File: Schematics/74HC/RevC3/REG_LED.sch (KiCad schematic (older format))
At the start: 224 parts

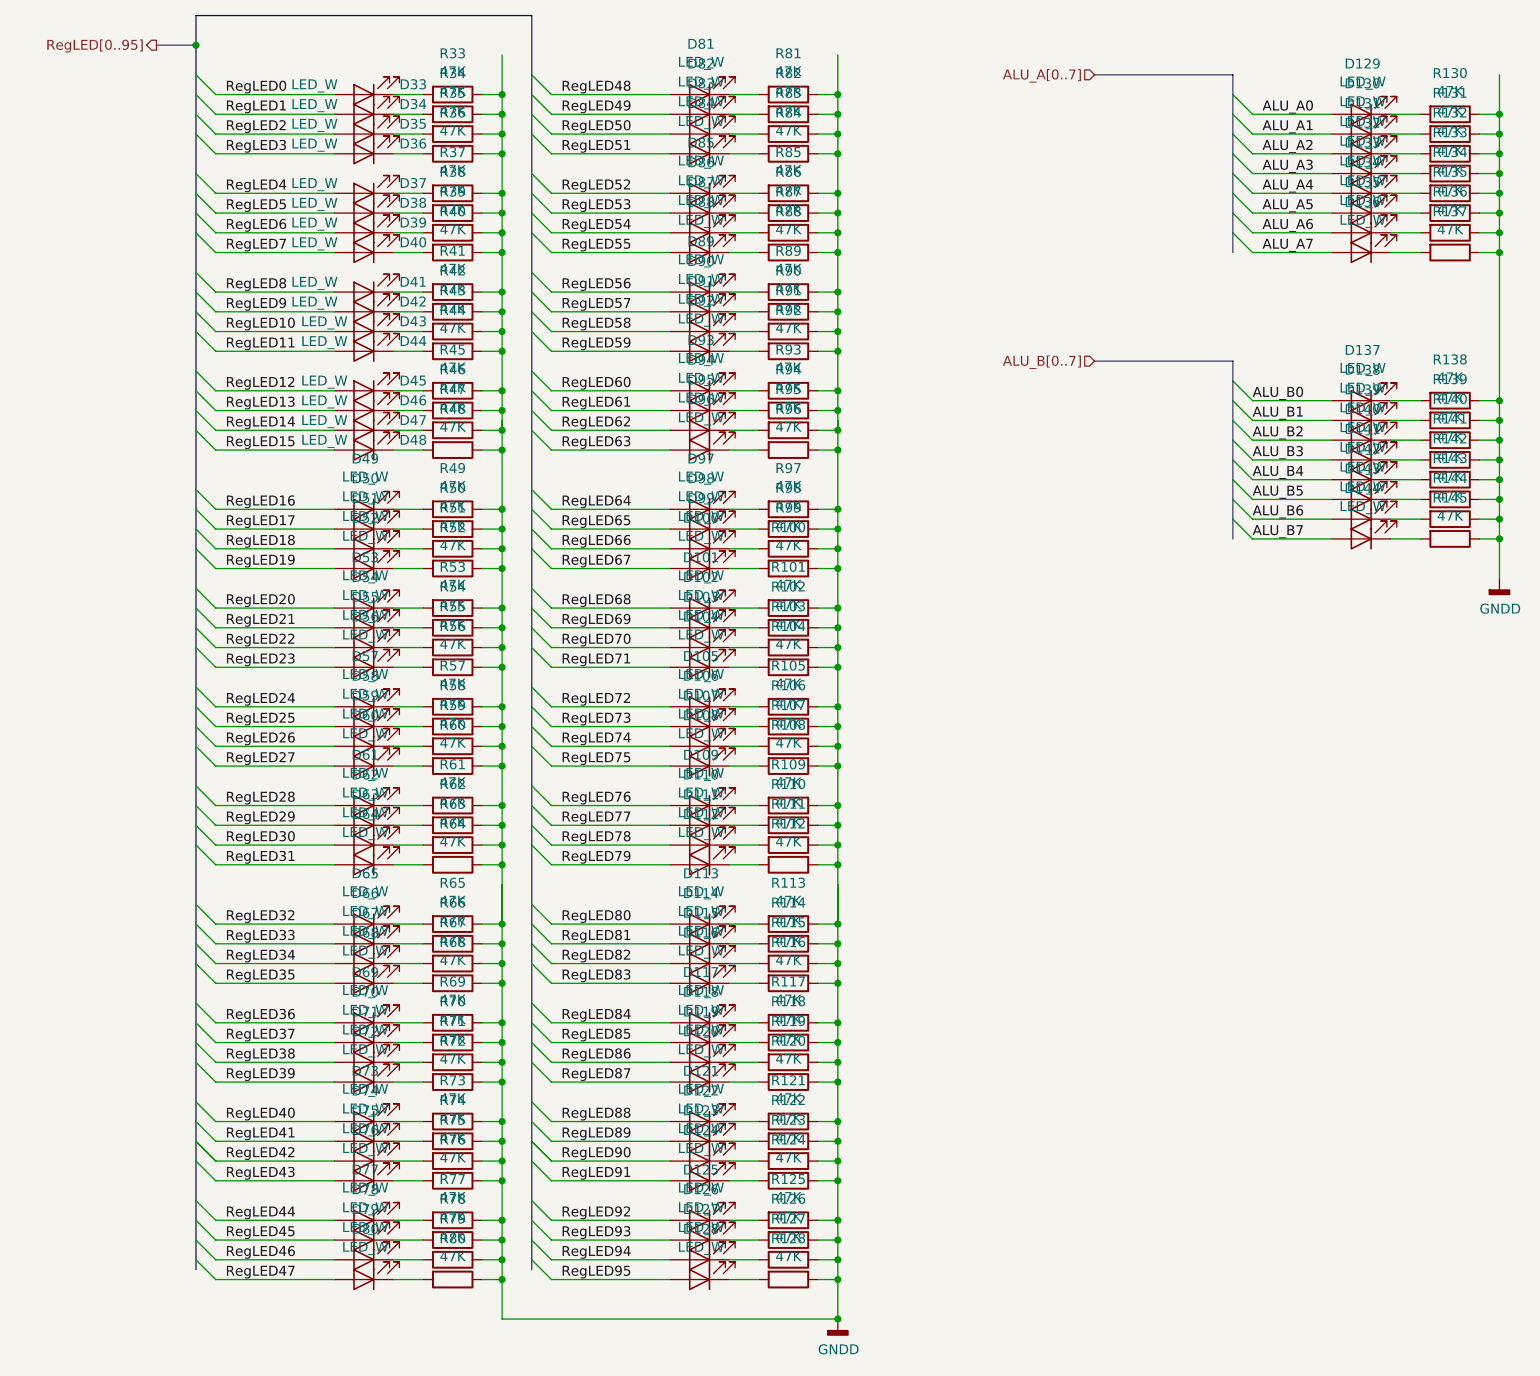
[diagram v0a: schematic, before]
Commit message: revA3
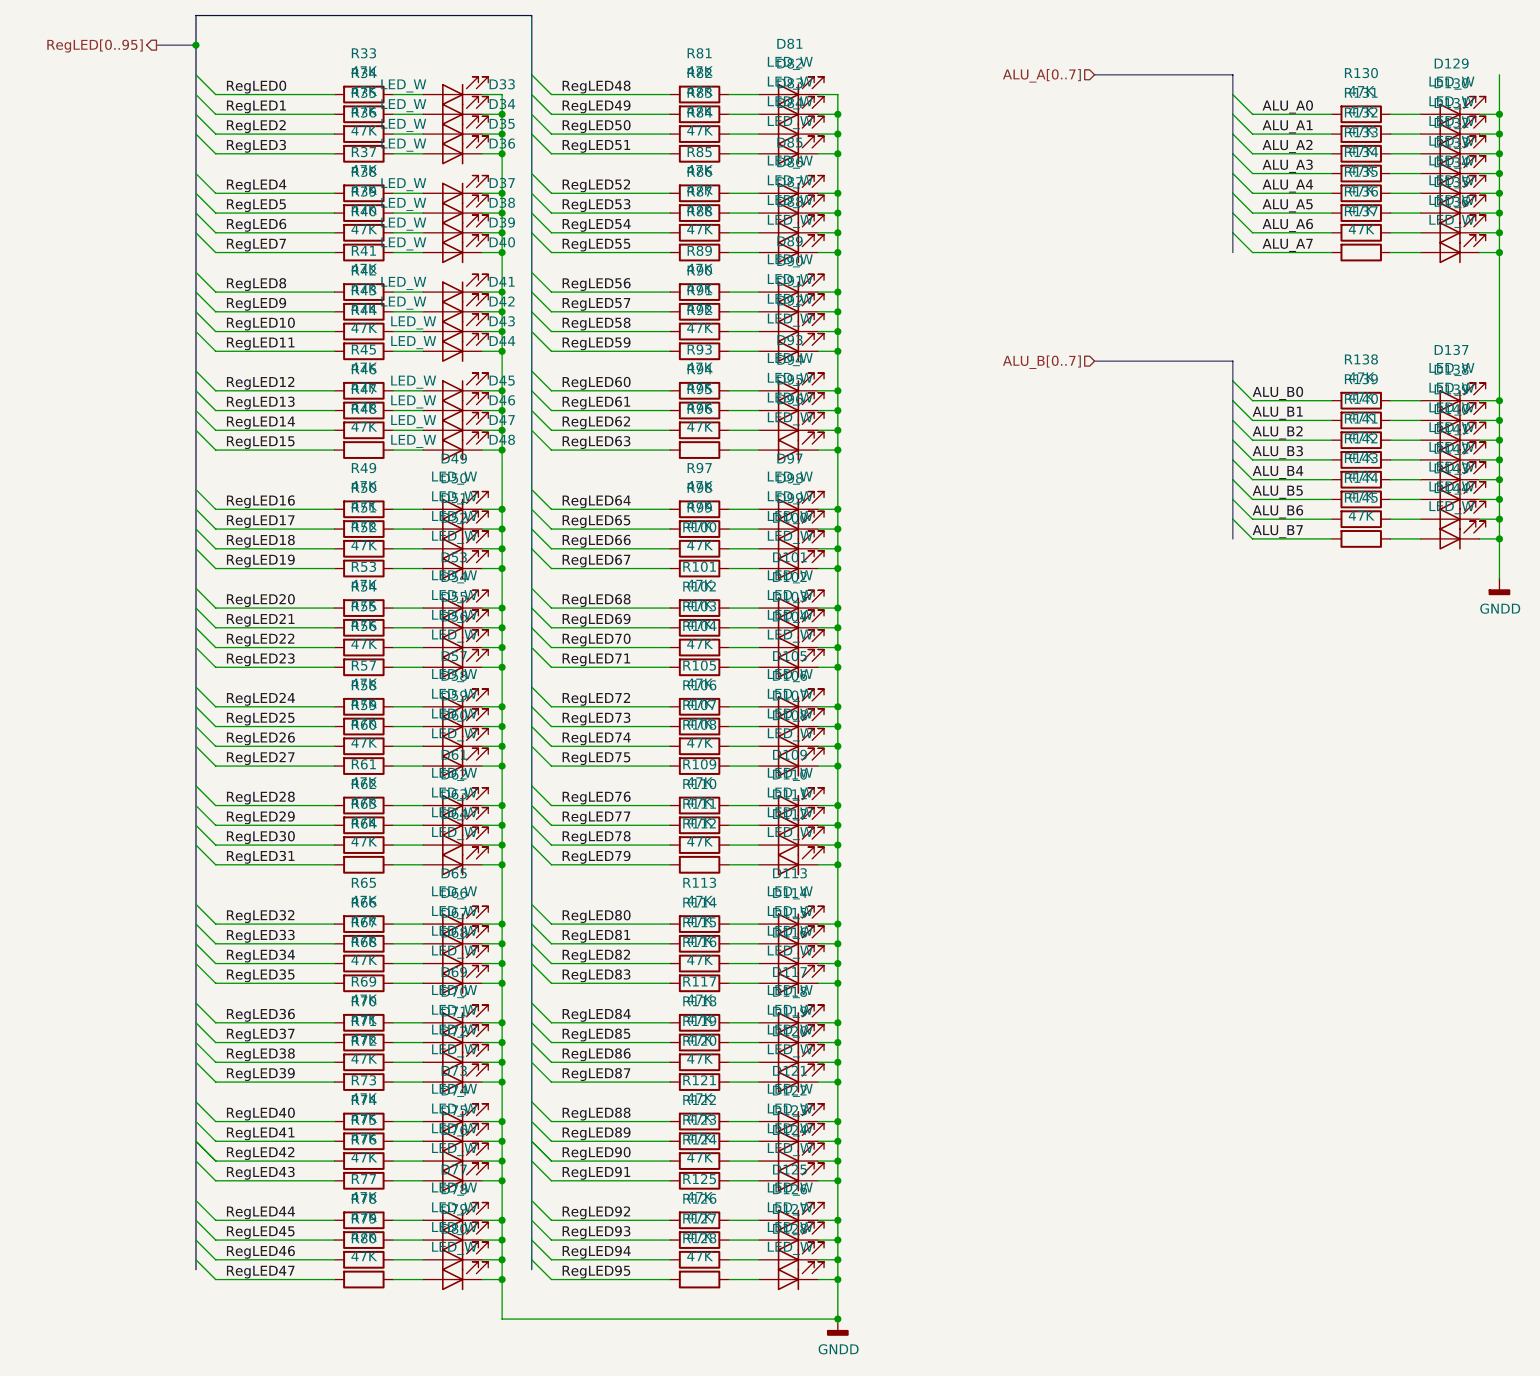
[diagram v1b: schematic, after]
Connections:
- net ALU_A0: now also R130.2; no longer D129.2 (A)
- net ALU_A1: now also R131.2; no longer D130.2 (A)
- net ALU_A2: now also R132.2; no longer D131.2 (A)
- net ALU_A3: now also R133.2; no longer D132.2 (A)
- net ALU_A4: now also R134.2; no longer D133.2 (A)
- net ALU_A5: now also R135.2; no longer D134.2 (A)
- net ALU_A6: now also R136.2; no longer D135.2 (A)
- net ALU_A7: now also R137.2; no longer D136.2 (A)
- net ALU_B0: now also R138.2; no longer D137.2 (A)
- net ALU_B1: now also R139.2; no longer D138.2 (A)
- net ALU_B2: now also R140.2; no longer D139.2 (A)
- net ALU_B3: now also R141.2; no longer D140.2 (A)
- net ALU_B4: now also R142.2; no longer D141.2 (A)
- net ALU_B5: now also R143.2; no longer D142.2 (A)
- net ALU_B6: now also R144.2; no longer D143.2 (A)
- net ALU_B7: now also R145.2; no longer D144.2 (A)
- net GNDD: now also D100.1 (K), D101.1 (K), D102.1 (K), D103.1 (K), D104.1 (K), D105.1 (K), D106.1 (K), D107.1 (K), D108.1 (K), D109.1 (K), D110.1 (K), D111.1 (K), D112.1 (K), D113.1 (K), D114.1 (K), D115.1 (K), D116.1 (K), D117.1 (K), D118.1 (K), D119.1 (K), D120.1 (K), D121.1 (K), D122.1 (K), D123.1 (K), D124.1 (K), D125.1 (K), D126.1 (K), D127.1 (K), D128.1 (K), D129.1 (K), D130.1 (K), D131.1 (K), D132.1 (K), D133.1 (K), D134.1 (K), D135.1 (K), D136.1 (K), D137.1 (K), D138.1 (K), D139.1 (K), D140.1 (K), D141.1 (K), D142.1 (K), D143.1 (K), D144.1 (K), D33.1 (K), D34.1 (K), D35.1 (K), D36.1 (K), D37.1 (K), D38.1 (K), D39.1 (K), D40.1 (K), D41.1 (K), D42.1 (K), D43.1 (K), D44.1 (K), D45.1 (K), D46.1 (K), D47.1 (K), D48.1 (K), D49.1 (K), D50.1 (K), D51.1 (K), D52.1 (K), D53.1 (K), D54.1 (K), D55.1 (K), D56.1 (K), D57.1 (K), D58.1 (K), D59.1 (K), D60.1 (K), D61.1 (K), D62.1 (K), D63.1 (K), D64.1 (K), D65.1 (K), D66.1 (K), D67.1 (K), D68.1 (K), D69.1 (K), D70.1 (K), D71.1 (K), D72.1 (K), D73.1 (K), D74.1 (K), D75.1 (K), D76.1 (K), D77.1 (K), D78.1 (K), D79.1 (K), D80.1 (K), D81.1 (K), D82.1 (K), D83.1 (K), D84.1 (K), D85.1 (K), D86.1 (K), D87.1 (K), D88.1 (K), D89.1 (K), D90.1 (K), D91.1 (K), D92.1 (K), D93.1 (K), D94.1 (K), D95.1 (K), D96.1 (K), D97.1 (K), D98.1 (K), D99.1 (K); no longer R100.1, R101.1, R102.1, R103.1, R104.1, R105.1, R106.1, R107.1, R108.1, R109.1, R110.1, R111.1, R112.1, R113.1, R114.1, R115.1, R116.1, R117.1, R118.1, R119.1, R120.1, R121.1, R122.1, R123.1, R124.1, R125.1, R126.1, R127.1, R128.1, R130.1, R131.1, R132.1, R133.1, R134.1, R135.1, R136.1, R137.1, R138.1, R139.1, R140.1, R141.1, R142.1, R143.1, R144.1, R145.1, R33.1, R34.1, R35.1, R36.1, R37.1, R38.1, R39.1, R40.1, R41.1, R42.1, R43.1, R44.1, R45.1, R46.1, R47.1, R48.1, R49.1, R50.1, R51.1, R52.1, R53.1, R54.1, R55.1, R56.1, R57.1, R58.1, R59.1, R60.1, R61.1, R62.1, R63.1, R64.1, R65.1, R66.1, R67.1, R68.1, R69.1, R70.1, R71.1, R72.1, R73.1, R74.1, R75.1, R76.1, R77.1, R78.1, R79.1, R80.1, R81.1, R82.1, R83.1, R84.1, R85.1, R86.1, R87.1, R88.1, R89.1, R90.1, R91.1, R92.1, R93.1, R94.1, R95.1, R96.1, R97.1, R98.1, R99.1
- net RegLED0: now also R33.2; no longer D33.2 (A)
- net RegLED1: now also R34.2; no longer D34.2 (A)
- net RegLED10: now also R43.2; no longer D43.2 (A)
- net RegLED11: now also R44.2; no longer D44.2 (A)
- net RegLED12: now also R45.2; no longer D45.2 (A)
- net RegLED13: now also R46.2; no longer D46.2 (A)
- net RegLED14: now also R47.2; no longer D47.2 (A)
- net RegLED15: now also R48.2; no longer D48.2 (A)
- net RegLED16: now also R49.2; no longer D49.2 (A)
- net RegLED17: now also R50.2; no longer D50.2 (A)
- net RegLED18: now also R51.2; no longer D51.2 (A)
- net RegLED19: now also R52.2; no longer D52.2 (A)
- net RegLED2: now also R35.2; no longer D35.2 (A)
- net RegLED20: now also R53.2; no longer D53.2 (A)
- net RegLED21: now also R54.2; no longer D54.2 (A)
- net RegLED22: now also R55.2; no longer D55.2 (A)
- net RegLED23: now also R56.2; no longer D56.2 (A)
- net RegLED24: now also R57.2; no longer D57.2 (A)
- net RegLED25: now also R58.2; no longer D58.2 (A)
- net RegLED26: now also R59.2; no longer D59.2 (A)
- net RegLED27: now also R60.2; no longer D60.2 (A)
- net RegLED28: now also R61.2; no longer D61.2 (A)
- net RegLED29: now also R62.2; no longer D62.2 (A)
- net RegLED3: now also R36.2; no longer D36.2 (A)
- net RegLED30: now also R63.2; no longer D63.2 (A)
- net RegLED31: now also R64.2; no longer D64.2 (A)
- net RegLED32: now also R65.2; no longer D65.2 (A)
- net RegLED33: now also R66.2; no longer D66.2 (A)
- net RegLED34: now also R67.2; no longer D67.2 (A)
- net RegLED35: now also R68.2; no longer D68.2 (A)
- net RegLED36: now also R69.2; no longer D69.2 (A)
- net RegLED37: now also R70.2; no longer D70.2 (A)
- net RegLED38: now also R71.2; no longer D71.2 (A)
- net RegLED39: now also R72.2; no longer D72.2 (A)
- net RegLED4: now also R37.2; no longer D37.2 (A)
- net RegLED40: now also R73.2; no longer D73.2 (A)
- net RegLED41: now also R74.2; no longer D74.2 (A)
- net RegLED42: now also R75.2; no longer D75.2 (A)
- net RegLED43: now also R76.2; no longer D76.2 (A)
- net RegLED44: now also R77.2; no longer D77.2 (A)
- net RegLED45: now also R78.2; no longer D78.2 (A)
- net RegLED46: now also R79.2; no longer D79.2 (A)
- net RegLED47: now also R80.2; no longer D80.2 (A)
- net RegLED48: now also R81.2; no longer D81.2 (A)
- net RegLED49: now also R82.2; no longer D82.2 (A)
- net RegLED5: now also R38.2; no longer D38.2 (A)
- net RegLED50: now also R83.2; no longer D83.2 (A)
- net RegLED51: now also R84.2; no longer D84.2 (A)
- net RegLED52: now also R85.2; no longer D85.2 (A)
- net RegLED53: now also R86.2; no longer D86.2 (A)
- net RegLED54: now also R87.2; no longer D87.2 (A)
- net RegLED55: now also R88.2; no longer D88.2 (A)
- net RegLED56: now also R89.2; no longer D89.2 (A)
- net RegLED57: now also R90.2; no longer D90.2 (A)
- net RegLED58: now also R91.2; no longer D91.2 (A)
- net RegLED59: now also R92.2; no longer D92.2 (A)
- net RegLED6: now also R39.2; no longer D39.2 (A)
- net RegLED60: now also R93.2; no longer D93.2 (A)
- net RegLED61: now also R94.2; no longer D94.2 (A)
- net RegLED62: now also R95.2; no longer D95.2 (A)
- net RegLED63: now also R96.2; no longer D96.2 (A)
- net RegLED64: now also R97.2; no longer D97.2 (A)
- net RegLED65: now also R98.2; no longer D98.2 (A)
- net RegLED66: now also R99.2; no longer D99.2 (A)
- net RegLED67: now also R100.2; no longer D100.2 (A)
- net RegLED68: now also R101.2; no longer D101.2 (A)
- net RegLED69: now also R102.2; no longer D102.2 (A)
- net RegLED7: now also R40.2; no longer D40.2 (A)
- net RegLED70: now also R103.2; no longer D103.2 (A)
- net RegLED71: now also R104.2; no longer D104.2 (A)
- net RegLED72: now also R105.2; no longer D105.2 (A)
- net RegLED73: now also R106.2; no longer D106.2 (A)
- net RegLED74: now also R107.2; no longer D107.2 (A)
- net RegLED75: now also R108.2; no longer D108.2 (A)
- net RegLED76: now also R109.2; no longer D109.2 (A)
- net RegLED77: now also R110.2; no longer D110.2 (A)
- net RegLED78: now also R111.2; no longer D111.2 (A)
- net RegLED79: now also R112.2; no longer D112.2 (A)
- net RegLED8: now also R41.2; no longer D41.2 (A)
- net RegLED80: now also R113.2; no longer D113.2 (A)
- net RegLED81: now also R114.2; no longer D114.2 (A)
- net RegLED82: now also R115.2; no longer D115.2 (A)
- net RegLED83: now also R116.2; no longer D116.2 (A)
- net RegLED84: now also R117.2; no longer D117.2 (A)
- net RegLED85: now also R118.2; no longer D118.2 (A)
- net RegLED86: now also R119.2; no longer D119.2 (A)
- net RegLED87: now also R120.2; no longer D120.2 (A)
- net RegLED88: now also R121.2; no longer D121.2 (A)
- net RegLED89: now also R122.2; no longer D122.2 (A)
- net RegLED9: now also R42.2; no longer D42.2 (A)
- net RegLED90: now also R123.2; no longer D123.2 (A)
- net RegLED91: now also R124.2; no longer D124.2 (A)
- net RegLED92: now also R125.2; no longer D125.2 (A)
- net RegLED93: now also R126.2; no longer D126.2 (A)
- net RegLED94: now also R127.2; no longer D127.2 (A)
- net RegLED95: now also R128.2; no longer D128.2 (A)
- new net: D129.2 (A), R130.1
- new net: D130.2 (A), R131.1
- new net: D131.2 (A), R132.1
- new net: D132.2 (A), R133.1
- new net: D137.2 (A), R138.1
- new net: D138.2 (A), R139.1
- new net: D139.2 (A), R140.1
- new net: D140.2 (A), R141.1
- new net: D141.2 (A), R142.1
- new net: D142.2 (A), R143.1
- new net: D143.2 (A), R144.1
- new net: D144.2 (A), R145.1
- new net: D133.2 (A), R134.1
- new net: D134.2 (A), R135.1
- new net: D135.2 (A), R136.1
- new net: D136.2 (A), R137.1
- new net: D33.2 (A), R33.1
- new net: D34.2 (A), R34.1
- new net: D35.2 (A), R35.1
- new net: D36.2 (A), R36.1
- new net: D37.2 (A), R37.1
- new net: D38.2 (A), R38.1
- new net: D39.2 (A), R39.1
- new net: D40.2 (A), R40.1
- new net: D41.2 (A), R41.1
- new net: D42.2 (A), R42.1
- new net: D43.2 (A), R43.1
- new net: D44.2 (A), R44.1
- new net: D45.2 (A), R45.1
- new net: D46.2 (A), R46.1
- new net: D47.2 (A), R47.1
- new net: D48.2 (A), R48.1
- new net: D49.2 (A), R49.1
- new net: D50.2 (A), R50.1
- new net: D51.2 (A), R51.1
- new net: D52.2 (A), R52.1
- new net: D53.2 (A), R53.1
- new net: D54.2 (A), R54.1
- new net: D55.2 (A), R55.1
- new net: D56.2 (A), R56.1
- new net: D57.2 (A), R57.1
- new net: D58.2 (A), R58.1
- new net: D59.2 (A), R59.1
- new net: D60.2 (A), R60.1
- new net: D61.2 (A), R61.1
- new net: D62.2 (A), R62.1
- new net: D63.2 (A), R63.1
- new net: D64.2 (A), R64.1
- new net: D65.2 (A), R65.1
- new net: D66.2 (A), R66.1
- new net: D67.2 (A), R67.1
- new net: D68.2 (A), R68.1
- new net: D69.2 (A), R69.1
- new net: D70.2 (A), R70.1
- new net: D71.2 (A), R71.1
- new net: D72.2 (A), R72.1
- new net: D73.2 (A), R73.1
- new net: D74.2 (A), R74.1
- new net: D75.2 (A), R75.1
- new net: D76.2 (A), R76.1
- new net: D77.2 (A), R77.1
- new net: D78.2 (A), R78.1
- new net: D79.2 (A), R79.1
- new net: D80.2 (A), R80.1
- new net: D113.2 (A), R113.1
- new net: D114.2 (A), R114.1
- new net: D115.2 (A), R115.1
- new net: D116.2 (A), R116.1
- new net: D117.2 (A), R117.1
- new net: D118.2 (A), R118.1
- new net: D119.2 (A), R119.1
- new net: D120.2 (A), R120.1
- new net: D121.2 (A), R121.1
- new net: D122.2 (A), R122.1
- new net: D123.2 (A), R123.1
- new net: D124.2 (A), R124.1
- new net: D125.2 (A), R125.1
- new net: D126.2 (A), R126.1
- new net: D127.2 (A), R127.1
- new net: D128.2 (A), R128.1
- new net: D97.2 (A), R97.1
- new net: D98.2 (A), R98.1
- new net: D99.2 (A), R99.1
- new net: D100.2 (A), R100.1
- new net: D101.2 (A), R101.1
- new net: D102.2 (A), R102.1
- new net: D103.2 (A), R103.1
- new net: D104.2 (A), R104.1
- new net: D105.2 (A), R105.1
- new net: D106.2 (A), R106.1
- new net: D107.2 (A), R107.1
- new net: D108.2 (A), R108.1
- new net: D109.2 (A), R109.1
- new net: D110.2 (A), R110.1
- new net: D111.2 (A), R111.1
- new net: D112.2 (A), R112.1
- new net: D81.2 (A), R81.1
- new net: D82.2 (A), R82.1
- new net: D83.2 (A), R83.1
- new net: D84.2 (A), R84.1
- new net: D85.2 (A), R85.1
- new net: D86.2 (A), R86.1
- new net: D87.2 (A), R87.1
- new net: D88.2 (A), R88.1
- new net: D89.2 (A), R89.1
- new net: D90.2 (A), R90.1
- new net: D91.2 (A), R91.1
- new net: D92.2 (A), R92.1
- new net: D93.2 (A), R93.1
- new net: D94.2 (A), R94.1
- new net: D95.2 (A), R95.1
- new net: D96.2 (A), R96.1
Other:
- moved on the sheet: D100, D101, D102, D103, D104, D105, D106, D107, D108, D109, D110, D111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
